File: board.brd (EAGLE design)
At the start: 92.1 x 90.5 mm, 64 parts, among them K1 FTR-K1C, K2 FTR-K1C, K3 FTR-K1C, K4 FTR-K1C, X6 PN61729-S

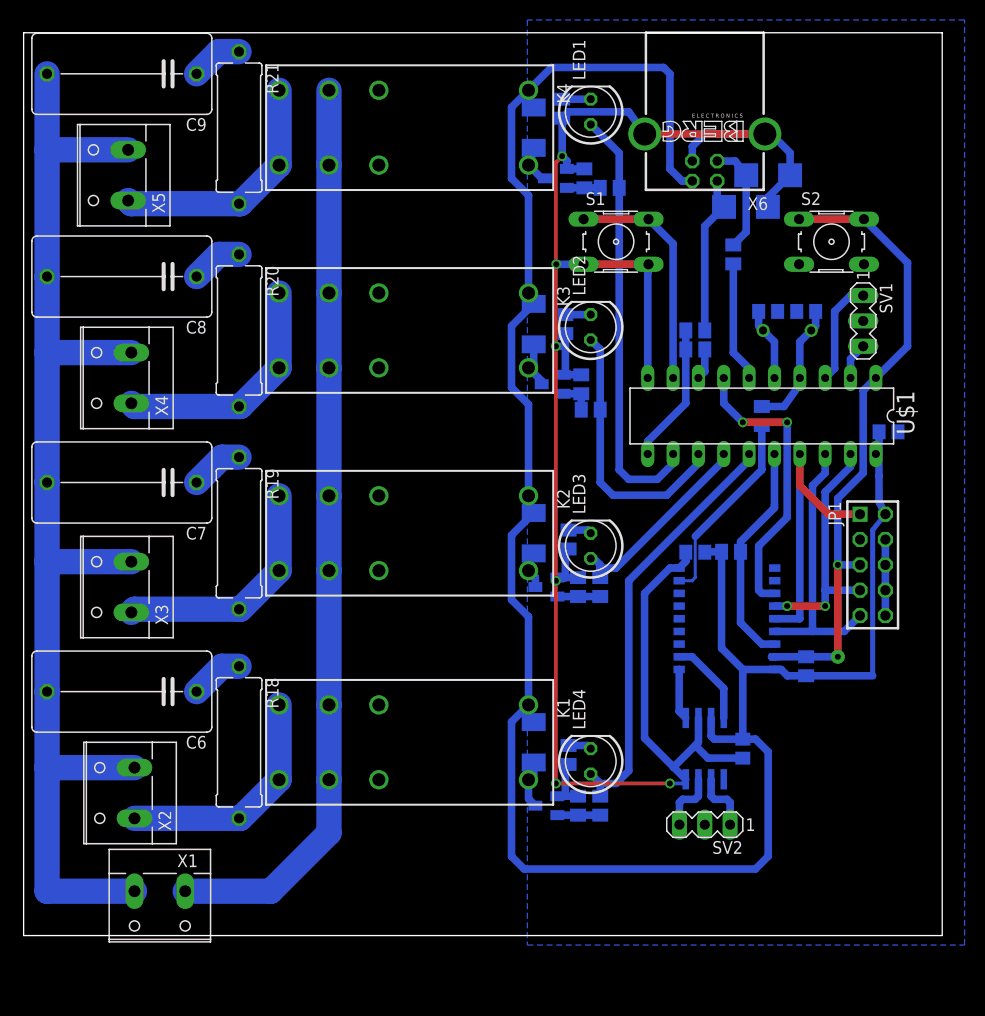
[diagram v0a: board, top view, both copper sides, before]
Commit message: fixing the fixing
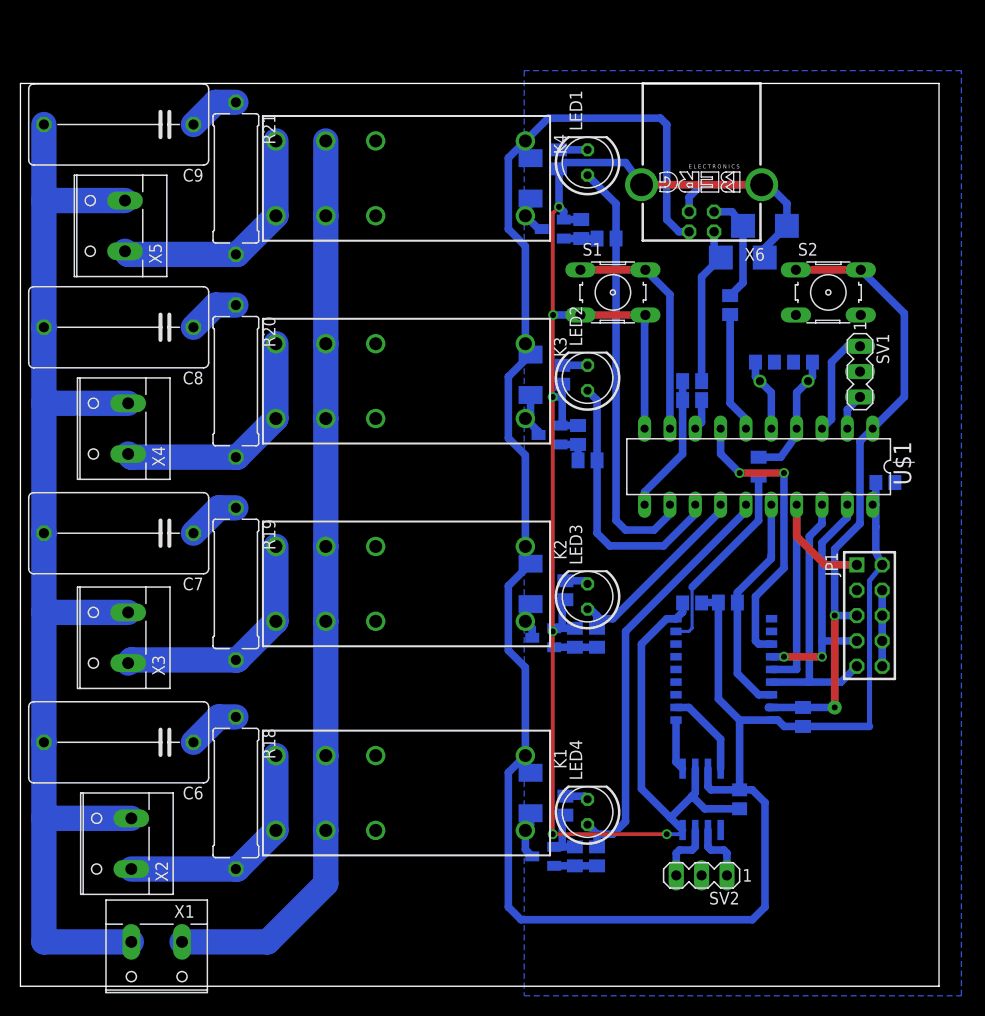
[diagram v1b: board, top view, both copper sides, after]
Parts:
- moved R7 5.09 mm to (56.2, 75.9)
- moved T4 5.09 mm to (53.3, 75.9)
- moved D2 5.09 mm to (51.1, 40.3)
- moved R19 5.09 mm to (21.6, 40.3)
- moved R3 5.09 mm to (55.6, 34.9)
- moved R4 5.09 mm to (57.8, 34.9)
- moved T3 5.09 mm to (53.0, 55.2)
- moved X3 5.09 mm to (10.2, 34.9)
- moved C4 5.09 mm to (67.3, 38.4)
- moved K2 5.09 mm to (38.1, 40.3)
- moved LED2 5.09 mm to (56.8, 61.0)
- moved R13 5.09 mm to (67.3, 58.7)
- moved R5 5.09 mm to (55.9, 55.2)
- moved T2 5.09 mm to (52.4, 34.9)
- moved D1 5.09 mm to (51.1, 19.4)
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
